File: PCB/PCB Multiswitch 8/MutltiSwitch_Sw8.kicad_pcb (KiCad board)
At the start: 2 copper layers, 10 parts, among them IC1 ATTINY84-P, IC2 ULN2803, P1 OUTPUT_1-8, P8 XANY_INPUT, X1 16Mhz

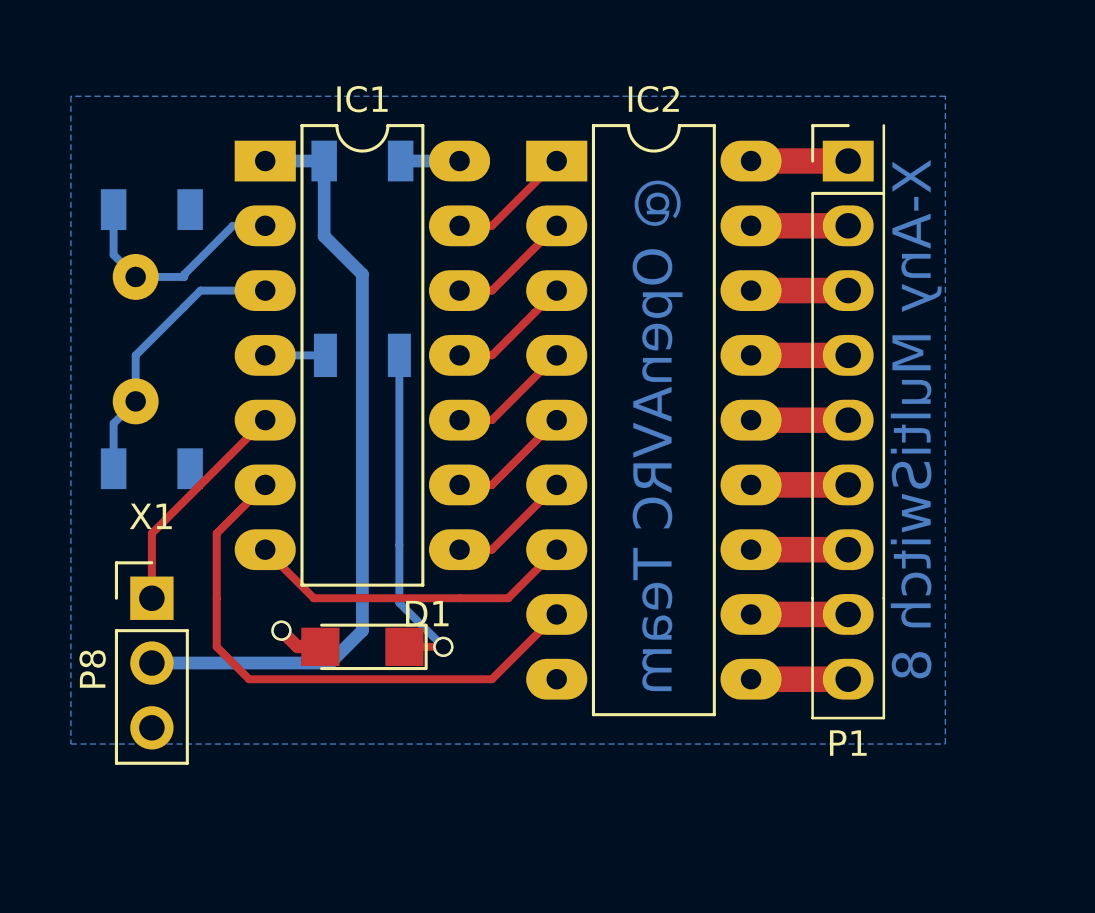
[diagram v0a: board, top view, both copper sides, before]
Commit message: Update_PCB-Multiswitch_8
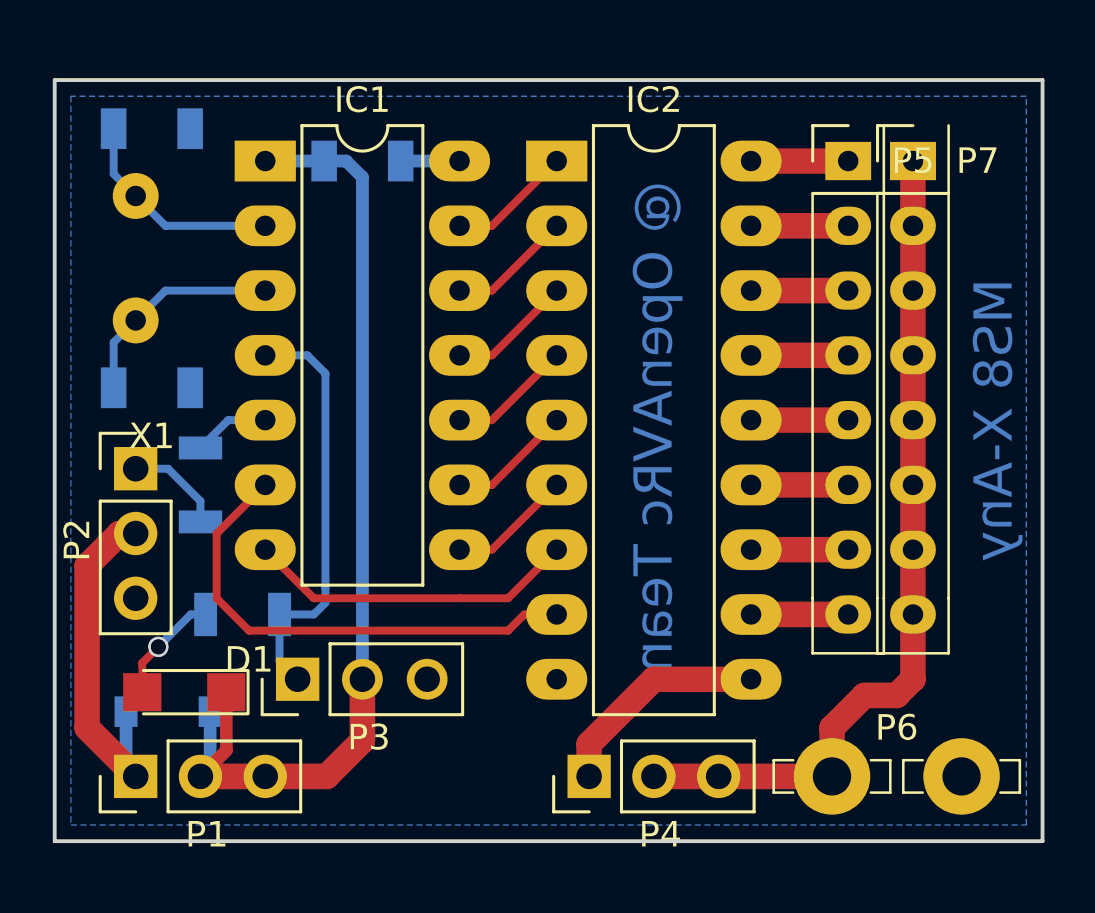
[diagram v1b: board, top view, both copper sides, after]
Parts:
- removed P8: XANY_INPUT, Pin_Header_Straight_1x03_Pitch2.54mm
- added D2: LL4148, D_SOD-123, B.Cu at (137.8, 113.0)
- added P2: XANY_INPUT, Pin_Header_Straight_1x03_Pitch2.54mm, F.Cu at (136.5, 103.5)
- added P3: SERVO, Pin_Header_Straight_1x03_Pitch2.54mm, F.Cu at (142.9, 111.8)
- added P4: SEL_ALIM, Pin_Header_Straight_1x03_Pitch2.54mm, F.Cu at (154.3, 115.6)
- added P5: OUTPUT_1X8, Pin_Header_Straight_1x09_Pitch2.54mm, F.Cu at (164.5, 91.4)
- added P6: VExt, Faston_V-5_08, F.Cu at (166.4, 115.6)
- added P7: OUTPUT_1X8_ALIM, Pin_Header_Straight_1x09_Pitch2.54mm, F.Cu at (167.0, 91.4)
- added R1: 1K, R_1206, B.Cu at (139.1, 104.1)
- P1: value OUTPUT_1-8 -> +V=VRx / +V<VRx; footprint Pin_Header_Straight_1x09_Pitch2.54mm -> Pin_Header_Straight_1x03_Pitch2.54mm
- R2: value 470 -> 330
- moved P1 36.9 mm to (136.5, 115.6), turned to 90 degrees
- moved R2 11.2 mm to (140.7, 109.2), turned to 180 degrees
- moved D1 7.21 mm to (138.4, 112.3)
- moved C2 3.17 mm to (137.2, 100.3)
- moved C3 3.17 mm to (137.2, 90.2)
- moved X1 3.17 mm to (136.5, 95.2)
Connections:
- D1 pad 1: Net-(D1-Pad1) -> +5V
- D1 pad 2: GND -> Net-(D1-Pad2)
- P1 pad 1: Net-(IC2-Pad18) -> +6V
- P1 pad 2: Net-(IC2-Pad17) -> +5V
- P1 pad 3: Net-(IC2-Pad16) -> +5V
- R2 pad 2: Net-(D1-Pad1) -> Net-(D1-Pad2)
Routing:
- net Net-(P4-Pad2): track 0.00 -> 33.2 mm
- net +6V: track 0.00 -> 14.2 mm
- net Net-(IC1-Pad4): track 2.36 -> 16.5 mm
- net Net-(D1-Pad1): track 13.7 -> 0.00 mm, vias 1 -> 0
- net +5V: track 30.1 -> 39.5 mm
- net Net-(IC1-Pad5): track 8.83 -> 2.99 mm
- net Net-(IC2-Pad10): track 3.81 -> 8.67 mm
- net Net-(D1-Pad2): track 0.00 -> 4.42 mm, vias 0 -> 1
- net Net-(P2-Pad1): track 0.00 -> 3.88 mm
- net Net-(IC1-Pad6): track 22.1 -> 19.4 mm
- net Net-(C2-Pad1): track 10.9 -> 8.56 mm
- net GND: track 4.10 -> 2.31 mm, vias 1 -> 0
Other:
- board outline added: 38.7 x 29.8 mm
- board text added: "@ OpenAVRc Team"
- board text added: "MS8 X-Any"
- board text removed: "@ OpenAVRC Team"
- board text removed: "X-Any MultiSwitch 8"
